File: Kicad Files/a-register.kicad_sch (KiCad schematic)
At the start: 20 parts, among them U26 74LS245, U27 74LS173, U28 74LS173

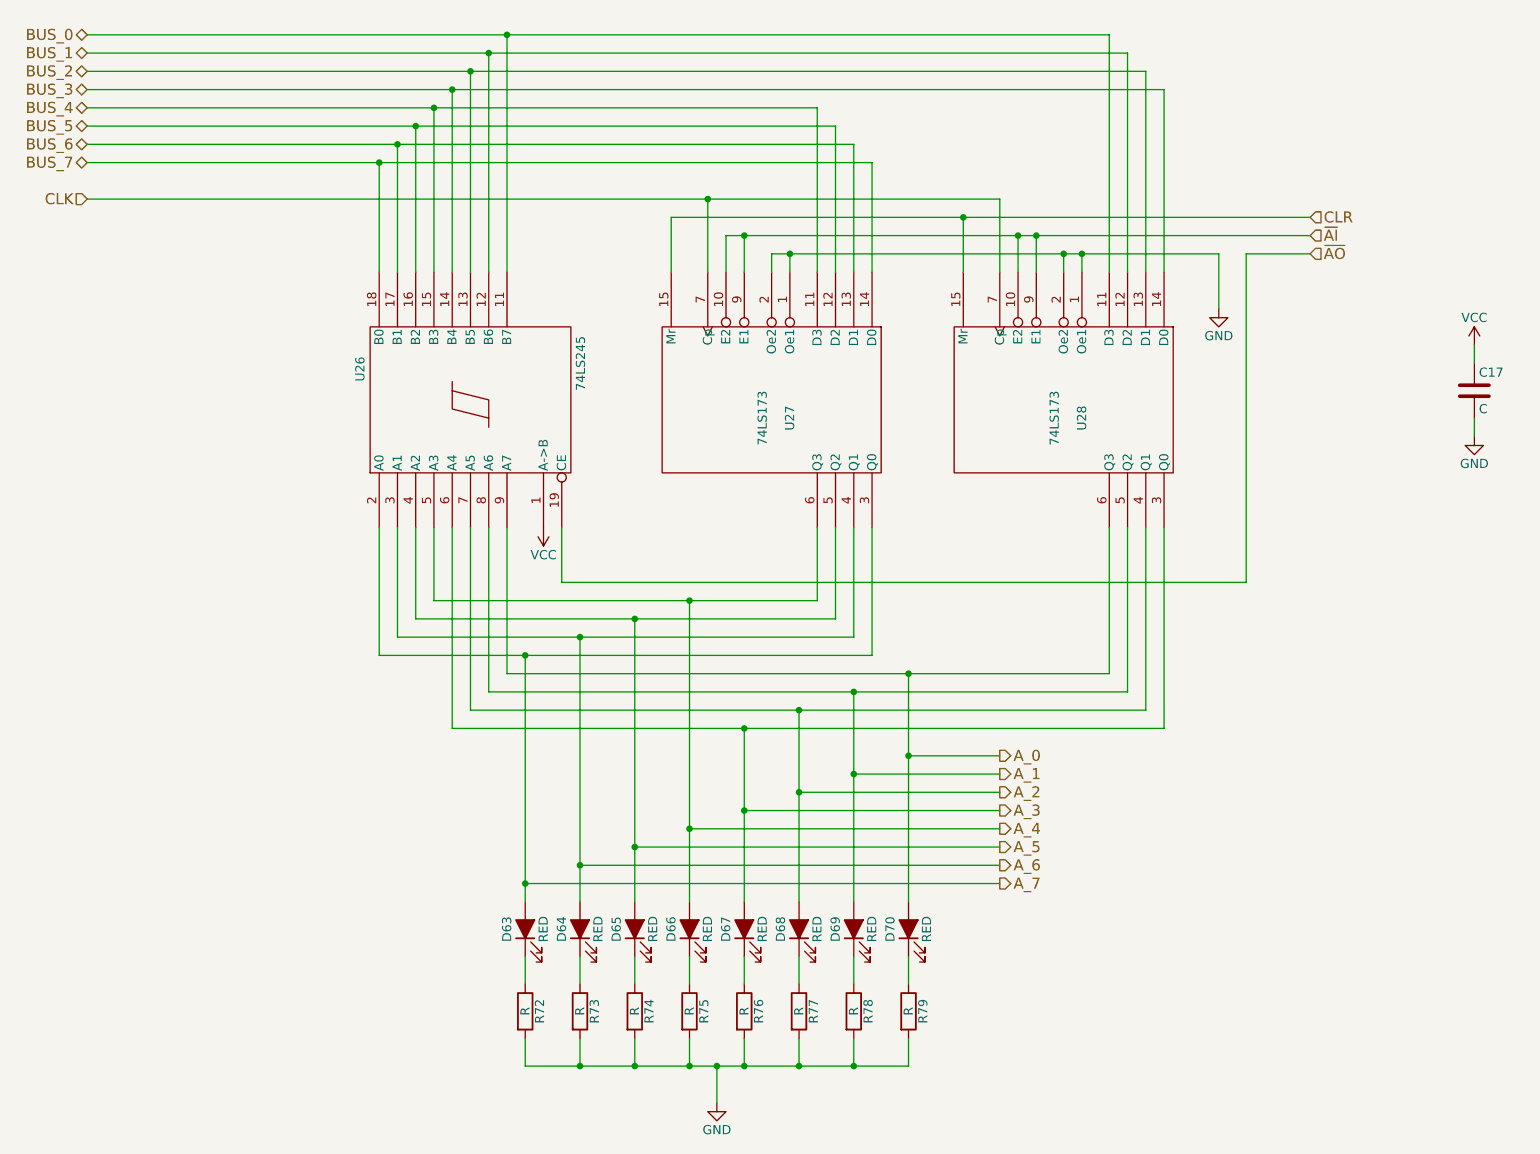
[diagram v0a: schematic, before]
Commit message: updated library
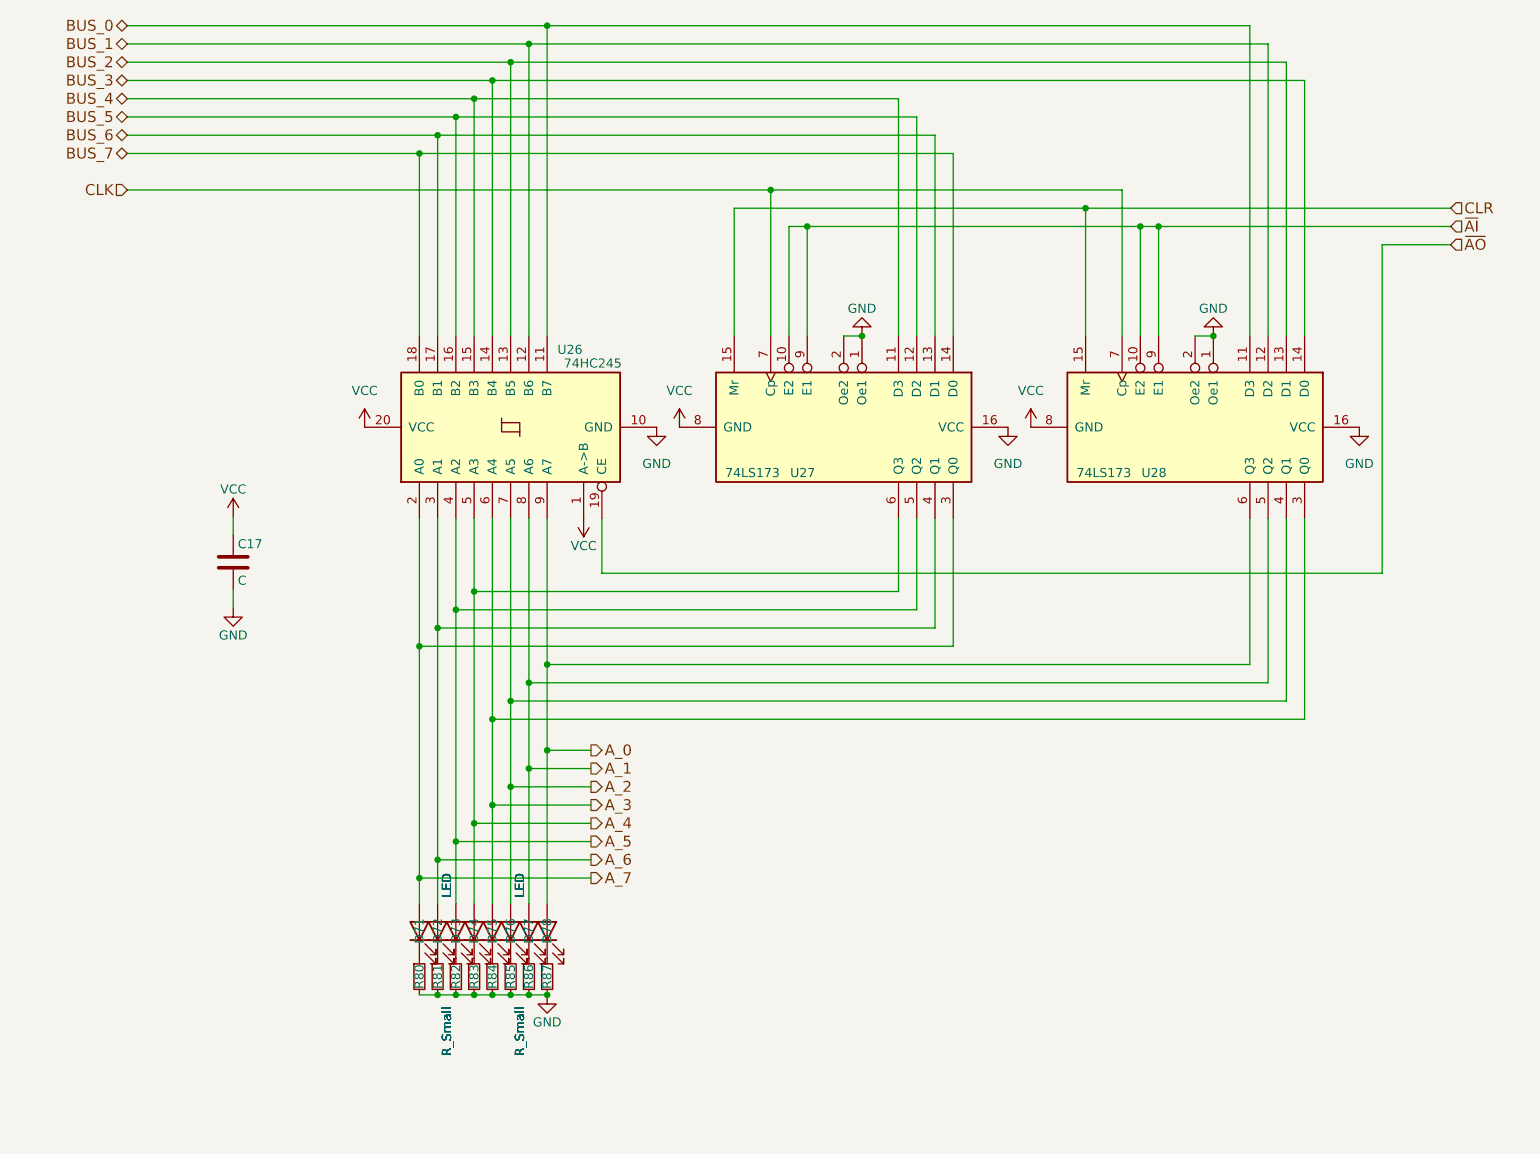
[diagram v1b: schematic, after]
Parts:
- removed D63, D64, D65, D66, D67, D68, D69, D70: RED, LED_THT:LED_D5.0mm, symbol 8bit-computer-rescue:LED_ALT-Device
- removed R72, R73, R74, R75, R76, R77, R78, R79: R, Resistor_THT:R_Axial_DIN0207_L6.3mm_D2.5mm_P7.62mm_Horizontal, symbol Device:R
- removed U26: 74LS245, Package_DIP:DIP-20_W7.62mm, symbol 8bit-computer-rescue:74LS245-8bit-computer-rescue
- removed U27, U28: 74LS173, Package_DIP:DIP-16_W7.62mm, symbol 8bit-computer-rescue:74LS173-8bit-computer-rescue
- added D71, D72, D73, D74, D75, D76, D77, D78: LED, symbol Device:LED
- added R80, R81, R82, R83, R84, R85, R86, R87: R_Small, symbol Device:R_Small
- added U26: 74HC245, symbol 74xx:74HC245
- added U27, U28: 74LS173, symbol 74xx:74LS173
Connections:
- net A_0: now also D78.2 (A), U26.9 (A7), U28.6 (Q3)
- net A_1: now also D77.2 (A), U26.8 (A6), U28.5 (Q2)
- net A_2: now also D76.2 (A), U26.7 (A5), U28.4 (Q1)
- net A_3: now also D75.2 (A), U26.6 (A4), U28.3 (Q0)
- net A_4: now also D74.2 (A), U26.5 (A3), U27.6 (Q3)
- net A_5: now also D73.2 (A), U26.4 (A2), U27.5 (Q2)
- net A_6: now also D72.2 (A), U26.3 (A1), U27.4 (Q1)
- net A_7: now also D71.2 (A), U26.2 (A0), U27.3 (Q0)
- net BUS_0: now also U26.11 (B7), U28.11 (D3)
- net BUS_1: now also U26.12 (B6), U28.12 (D2)
- net BUS_2: now also U26.13 (B5), U28.13 (D1)
- net BUS_3: now also U26.14 (B4), U28.14 (D0)
- net BUS_4: now also U26.15 (B3), U27.11 (D3)
- net BUS_5: now also U26.16 (B2), U27.12 (D2)
- net BUS_6: now also U26.17 (B1), U27.13 (D1)
- net BUS_7: now also U26.18 (B0), U27.14 (D0)
- net CLK: now also U27.7 (Cp), U28.7 (Cp)
- net CLR: now also U27.15 (Mr), U28.15 (Mr)
- net GND: now also R80.2, R81.2, R82.2, R83.2, R84.2, R85.2, R86.2, R87.2, U26.10 (GND), U27.1 (Oe1), U27.16 (VCC), U27.2 (Oe2), U28.1 (Oe1), U28.16 (VCC), U28.2 (Oe2)
- net VCC: now also U26.1 (A->B), U26.20 (VCC), U27.8 (GND), U28.8 (GND)
- net ~{AI}: now also U27.10 (E2), U27.9 (E1), U28.10 (E2), U28.9 (E1)
- net ~{AO}: now also U26.19 (CE)
- new net: D74.1 (K), R83.1
- new net: D73.1 (K), R82.1
- new net: D76.1 (K), R85.1
- new net: D71.1 (K), R80.1
- new net: D77.1 (K), R86.1
- new net: D72.1 (K), R81.1
- new net: D75.1 (K), R84.1
- new net: D78.1 (K), R87.1
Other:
- moved on the sheet: C17
